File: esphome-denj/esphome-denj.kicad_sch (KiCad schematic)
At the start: 20 parts

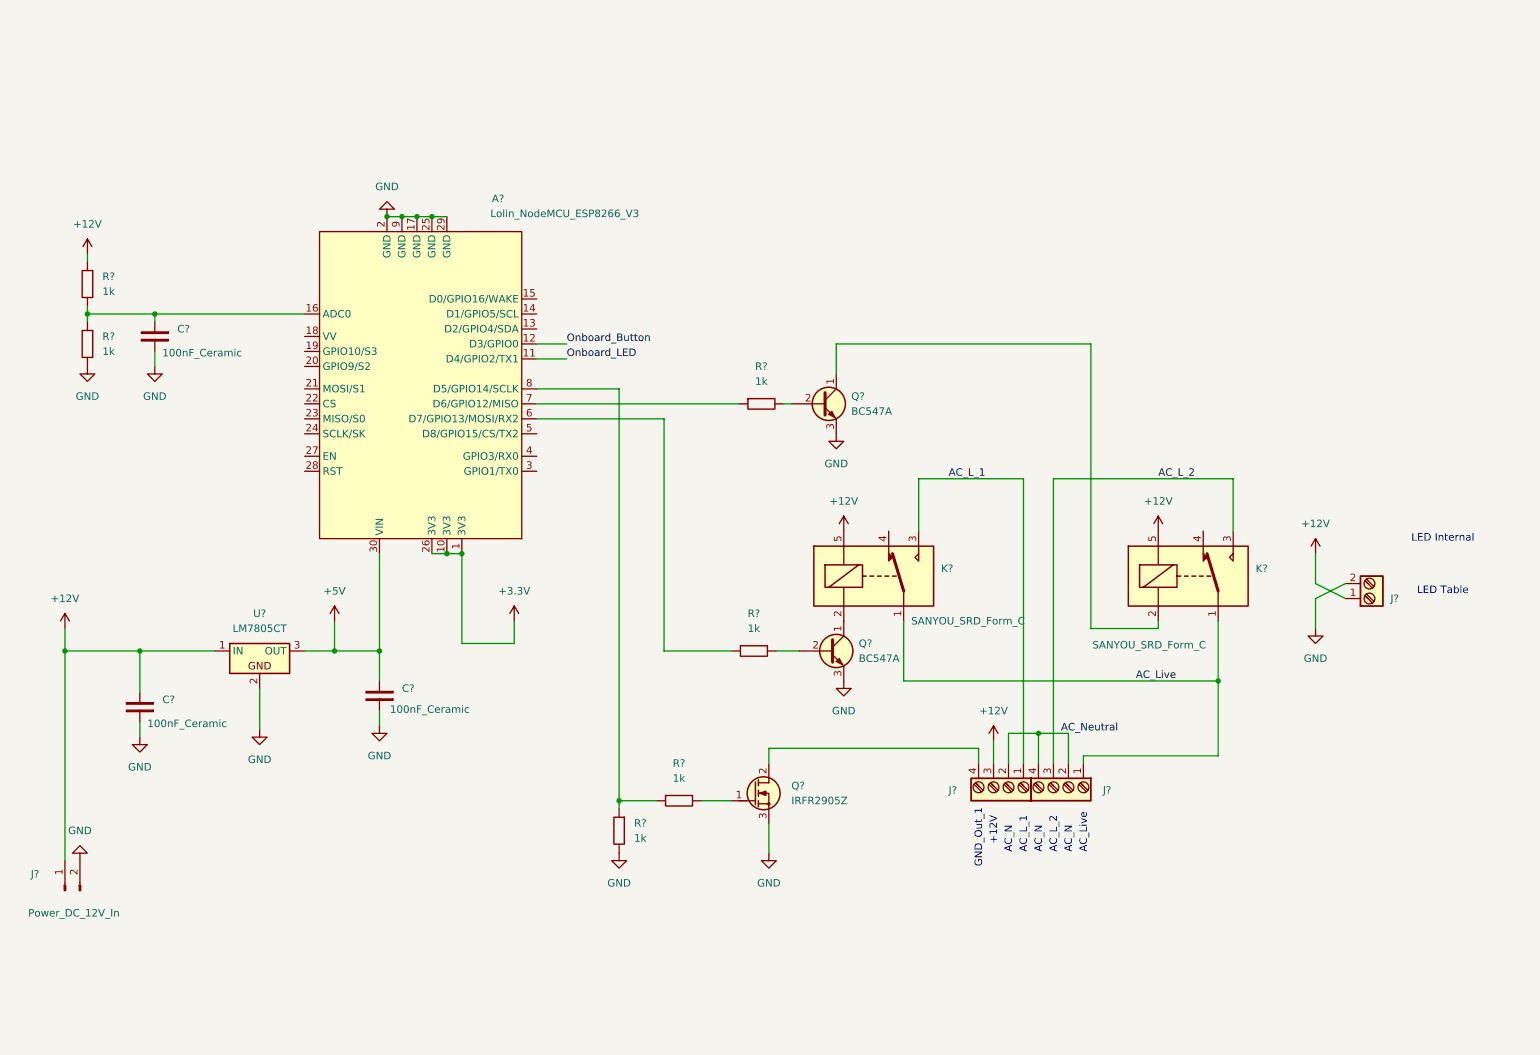
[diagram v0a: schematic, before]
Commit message: Denj V2 Schematic
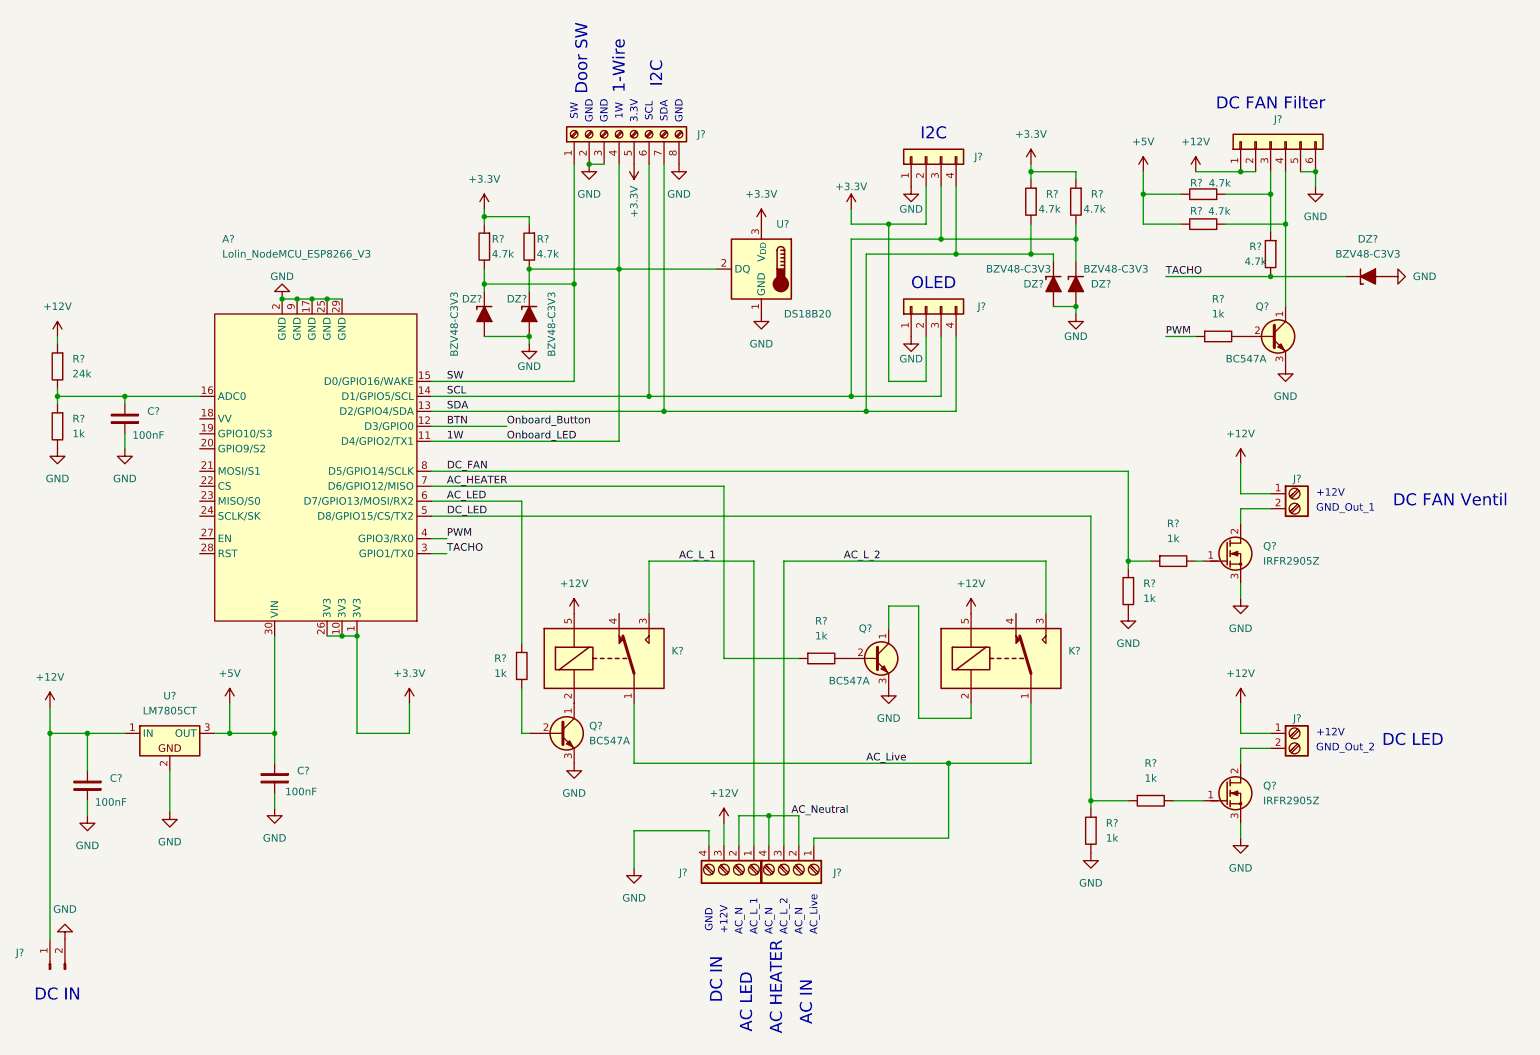
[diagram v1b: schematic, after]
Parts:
- removed Q?: IRFR2905Z, PCM_Package_TO_SOT_SMD_AKL:TO-252-2, symbol PCM_Transistor_MOSFET_AKL:IRFR2905Z
- removed R? (x3): 1k, Resistor_THT:R_Axial_DIN0207_L6.3mm_D2.5mm_P10.16mm_Horizontal, symbol PCM_SL_Resistors:1k
- added DZ? (x5): BZV48-C3V3, PCM_Diode_THT_AKL:D_DO-27_P15.24mm_Horizontal_Zener, symbol PCM_Diode_Zener_AKL:BZV48-C3V3
- added J? (x2): Conn_01x04, 4ms_Connector:Pins_1x04_2.54mm_TH_SWD, symbol PCM_4ms_Connector:Conn_01x04
- added J?: Screw_Terminal_01x08, symbol Connector:Screw_Terminal_01x08
- added J?: Conn_01x06, symbol Connector_Generic:Conn_01x06
- added J?: Screw_Terminal_2_P5.00mm, TerminalBlock_Phoenix:TerminalBlock_Phoenix_PT-1,5-2-5.0-H_1x02_P5.00mm_Horizontal, symbol PCM_SL_Screw_Terminal:Screw_Terminal_2_P5.00mm
- added Q? (x2): IRFR2905Z, PCM_Package_TO_SOT_SMD_AKL:TO-252-2, symbol PCM_Transistor_MOSFET_AKL:IRFR2905Z
- added Q?: BC547A, PCM_Package_TO_SOT_THT_AKL:TO-92_Inline_Wide_CBE, symbol PCM_Transistor_BJT_AKL:BC547A
- added R? (x7): 4.7k, Resistor_THT:R_Axial_DIN0207_L6.3mm_D2.5mm_P10.16mm_Horizontal, symbol PCM_SL_Resistors:1k
- added R? (x6): 1k, Resistor_THT:R_Axial_DIN0207_L6.3mm_D2.5mm_P10.16mm_Horizontal, symbol PCM_SL_Resistors:1k
- added U?: DS18B20, Package_TO_SOT_THT:TO-92_Inline, symbol Sensor_Temperature:DS18B20
- C? (x3): value 100nF_Ceramic -> 100nF
- R?: value 1k -> 24k
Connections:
- net +12V: now also J?.1, J?.1 (Pin_1), J?.2 (Pin_2)
- net +3.3V: now also J?.2 (Pin_2), J?.2 (Pin_2), J?.5 (Pin_5), R?.1, R?.1, R?.1, R?.1, U?.3 (V_{DD})
- net +5V: now also R?.2, R?.2
- net GND: now also J?.4, DZ?.2 (A), DZ?.2 (A), DZ?.2 (A), DZ?.2 (A), DZ?.2 (A), J?.1 (Pin_1), J?.1 (Pin_1), J?.2 (Pin_2), J?.3 (Pin_3), J?.5 (Pin_5), J?.6 (Pin_6), J?.8 (Pin_8), Q?.3 (E), Q?.3 (S), Q?.3 (S), R?.2, R?.2, U?.1 (GND); no longer J?.2
- net AC_HEATER: now reaches A?.7 (D6/GPIO12/MISO), R?.1
- net at Q?.2 (B): now also R?.2
- net DC_FAN: now reaches A?.8 (D5/GPIO14/SCLK)
- net DC_FAN: now also R?.1, R?.1
- net AC_LED: now reaches A?.6 (D7/GPIO13/MOSI/RX2)
- net AC_LED: now also R?.1
- net SDA: now reaches A?.13 (D2/GPIO4/SDA)
- net SDA: now also DZ?.1 (K), J?.4 (Pin_4), J?.4 (Pin_4), J?.7 (Pin_7), R?.2
- net SCL: now reaches A?.14 (D1/GPIO5/SCL)
- net SCL: now also DZ?.1 (K), J?.3 (Pin_3), J?.3 (Pin_3), J?.6 (Pin_6), R?.2
- net SW: now reaches A?.15 (D0/GPIO16/WAKE)
- net SW: now also DZ?.1 (K), J?.1 (Pin_1), R?.2
- net TACHO: now reaches A?.3 (GPIO1/TX0)
- net TACHO: now also DZ?.1 (K), R?.2
- net PWM: now reaches A?.4 (GPIO3/RX0)
- net PWM: now also R?.1
- net DC_LED: now reaches A?.5 (D8/GPIO15/CS/TX2)
- net DC_LED: now also R?.1, R?.1
- net Onboard_Button renamed BTN
- net Onboard_LED renamed 1W
- net 1W: now also DZ?.1 (K), J?.4 (Pin_4), R?.2, U?.2 (DQ)
- new net: Q?.1 (G), R?.2 (x2)
- new net: J?.2, Q?.2 (D) (x2)
- new net: J?.3 (Pin_3), R?.1, R?.1
- new net: J?.4 (Pin_4), Q?.1 (C), R?.1
- new net: Q?.2 (B), R?.2
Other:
- note added: "1-Wire"
- note added: "1W"
- note added: "3.3V"
- note added: "AC HEATER"
- note added: "AC IN"
- note added: "AC LED"
- note added: "DC FAN Filter"
- note added: "DC FAN Ventil"
- note added: "DC IN"
- note added: "DC LED"
- note added: "Door SW"
- note added: "GND"
- note added: "GND_Out_2"
- note added: "I2C"
- note added: "OLED"
- note added: "SCL"
- note added: "SDA"
- note added: "SW"
- note removed: "LED Internal"
- note removed: "LED Table"
- moved on the sheet: A?, C?, J?, K?, Q?, R?, U?
